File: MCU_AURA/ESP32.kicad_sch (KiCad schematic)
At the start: 15 parts, among them J2 TC2050-IDC-430, U200 ESP32-S3-WROOM-1, U201 USBLC6-2SC6

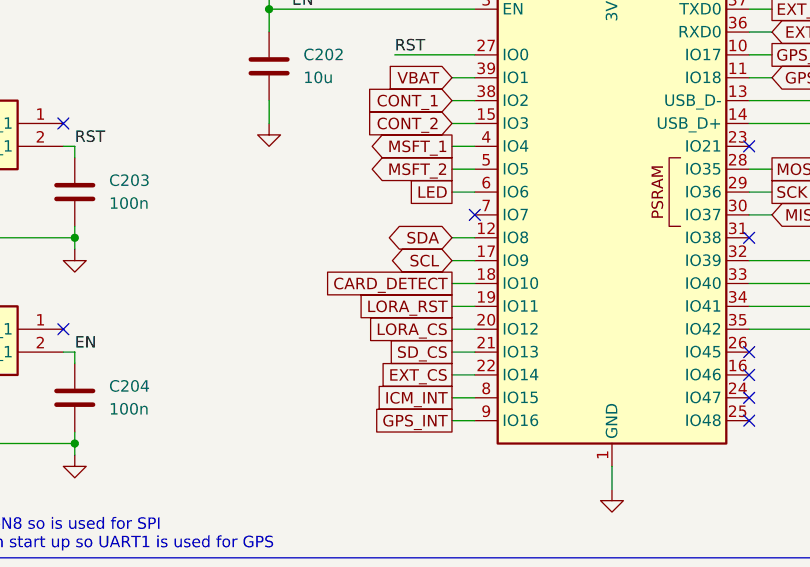
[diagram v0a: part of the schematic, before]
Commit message: Adding Connectors
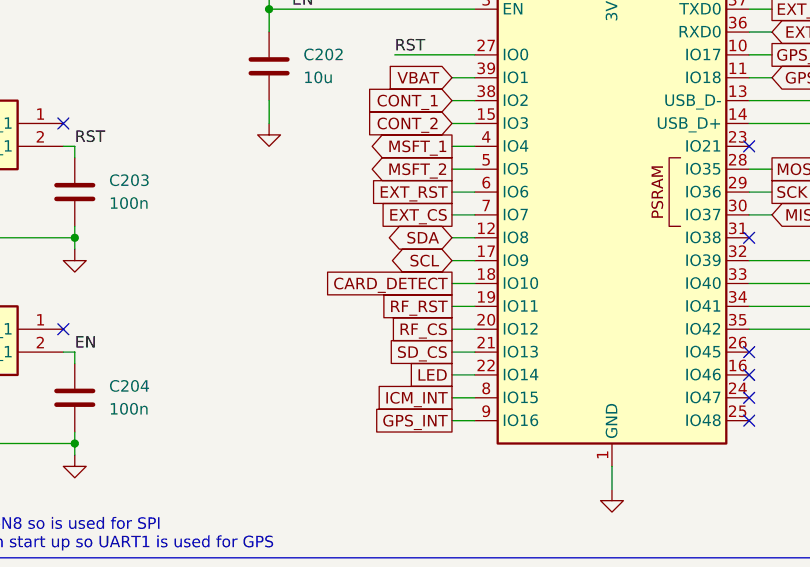
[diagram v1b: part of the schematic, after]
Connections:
- net EXT_CS: now also U200.7 (IO7); no longer U200.22 (IO14)
- net LED: now also U200.22 (IO14); no longer U200.6 (IO6)
- net LORA_CS renamed RF_CS
- net LORA_RST renamed RF_RST
- new net EXT_RST: U200.6 (IO6)
- no-connect marks 12 -> 11

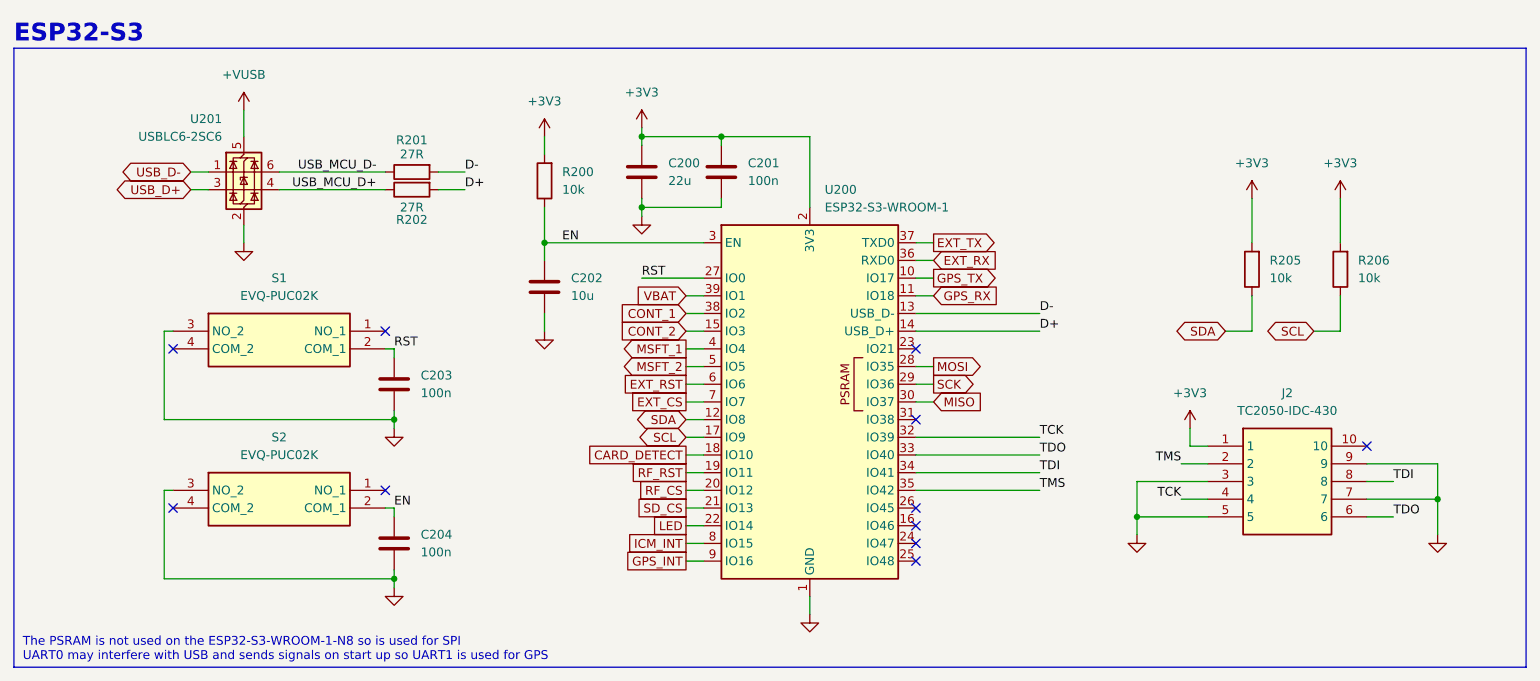
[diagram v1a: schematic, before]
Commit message: Initial Schematic Draft
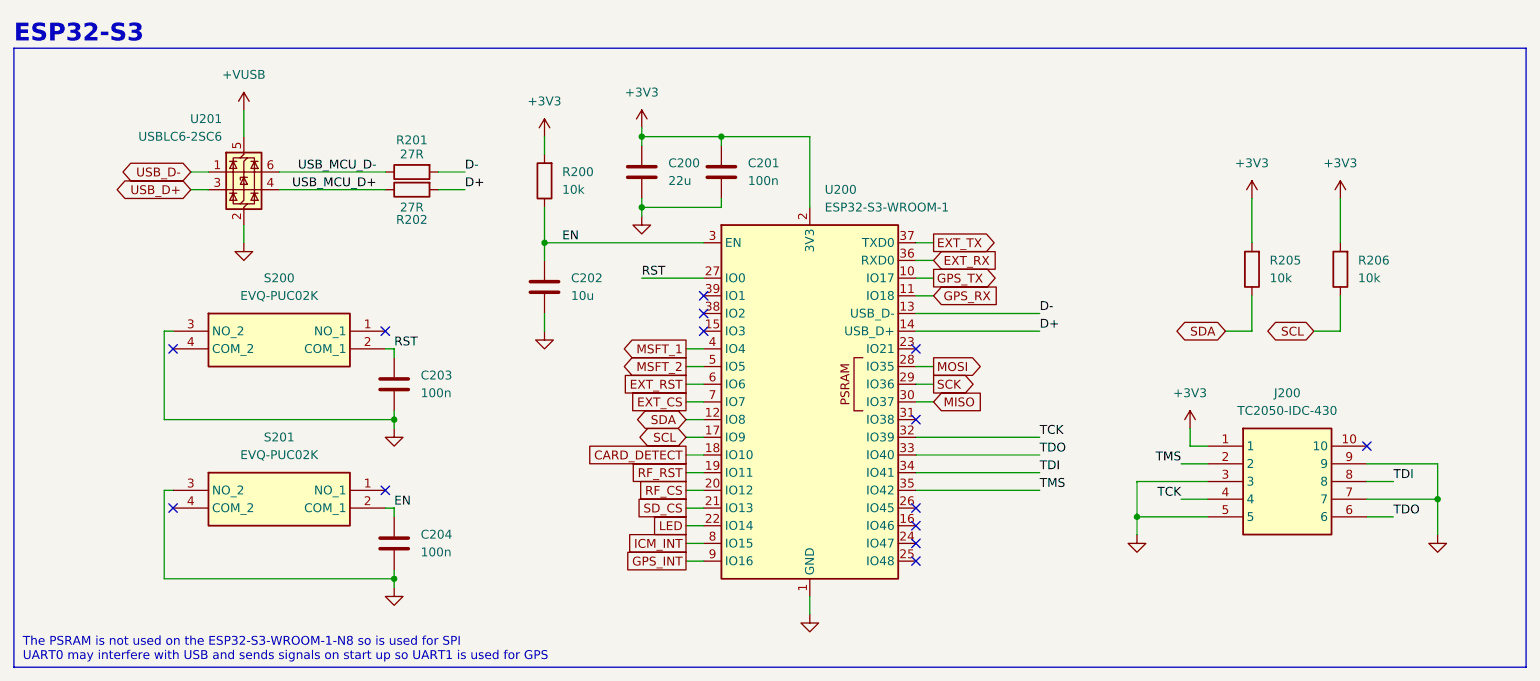
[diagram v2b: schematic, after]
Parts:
- renumbered J2 to J200, S1 to S200, S2 to S201
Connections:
- net CONT_1: no longer names the net of U200.38 (IO2)
- net CONT_2: no longer names the net of U200.15 (IO3)
- net VBAT: no longer names the net of U200.39 (IO1)
- no-connect marks 11 -> 14
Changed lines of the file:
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@@
 	)
 	(no_connect
+		(at 138.43 86.36)
+	)
+	(no_connect
+		(at 138.43 88.9)
+	)
+	(no_connect
 		(at 168.91 119.38)
 	)
@@
 	)
 	(no_connect
+		(at 138.43 91.44)
+	)
+	(no_connect
 		(at 168.91 104.14)
 	)
@@
 	(wire
 		(pts
-			(xy 135.89 91.44) (xy 138.43 91.44)
-		)
-		(stroke
-			(width 0)
-			(type default)
-		)
-	)
-	(wire
-		(pts
 			(xy 243.84 120.65) (xy 243.84 115.57)
 		)
@@
 	(wire
 		(pts
-			(xy 135.89 86.36) (xy 138.43 86.36)
-		)
-		(stroke
-			(width 0)
-			(type default)
-		)
-	)
-	(wire
-		(pts
-			(xy 135.89 88.9) (xy 138.43 88.9)
-		)
-		(stroke
-			(width 0)
-			(type default)
-		)
-	)
-	(wire
-		(pts
 			(xy 200.66 118.11) (xy 200.66 120.65)
 		)
@@
 		)
 	)
-	(global_label "CONT_1"
-		(shape input)
-		(at 135.89 88.9 180)
-		(fields_autoplaced yes)
-		(effects
-			(font
-				(size 1.27 1.27)
-			)
-			(justify right)
-		)
-		(property "Intersheetrefs" "${INTERSHEET_REFS}"
-			(at 125.8291 88.9 0)
-			(effects
-				(font
-					(size 1.27 1.27)
-				)
-				(justify right)
-				(hide yes)
-			)
-		)
-	)
 	(global_label "EXT_TX"
 		(shape output)
@@
 		)
 	)
-	(global_label "VBAT"
-		(shape input)
-		(at 135.89 86.36 180)
-		(fields_autoplaced yes)
-		(effects
-			(font
-				(size 1.27 1.27)
-			)
-			(justify right)
-		)
-		(property "Intersheetrefs" "${INTERSHEET_REFS}"
-			(at 128.49 86.36 0)
-			(effects
-				(font
-					(size 1.27 1.27)
-				)
-				(justify right)
-				(hide yes)
-			)
-		)
-	)
-	(global_label "CONT_2"
-		(shape input)
-		(at 135.89 91.44 180)
-		(fields_autoplaced yes)
-		(effects
-			(font
-				(size 1.27 1.27)
-			)
-			(justify right)
-		)
-		(property "Intersheetrefs" "${INTERSHEET_REFS}"
-			(at 125.8291 91.44 0)
-			(effects
-				(font
-					(size 1.27 1.27)
-				)
-				(justify right)
-				(hide yes)
-			)
-		)
-	)
 	(global_label "EXT_CS"
 		(shape passive)
@@
 		(dnp no)
 		(fields_autoplaced yes)
-		(property "Reference" "J2"
+		(property "Reference" "J200"
 			(at 222.25 100.33 0)
 			(effects
@@
 			(project ""
 				(path "/c0b09de1-c640-438f-9ef5-dda14a6aac71/b7286ff6-080d-4fe9-98ea-7dd25e1f4a61"
-					(reference "J2")
+					(reference "J200")
 					(unit 1)
 				)
@@
 		(dnp no)
 		(fields_autoplaced yes)
-		(property "Reference" "S1"
+		(property "Reference" "S200"
 			(at 77.47 83.82 0)
 			(effects
@@
 			(project ""
 				(path "/c0b09de1-c640-438f-9ef5-dda14a6aac71/b7286ff6-080d-4fe9-98ea-7dd25e1f4a61"
-					(reference "S1")
+					(reference "S200")
 					(unit 1)
 				)
@@
 		(dnp no)
 		(fields_autoplaced yes)
-		(property "Reference" "S2"
+		(property "Reference" "S201"
 			(at 77.47 106.68 0)
 			(effects
@@
 			(project "MCU_AURA"
 				(path "/c0b09de1-c640-438f-9ef5-dda14a6aac71/b7286ff6-080d-4fe9-98ea-7dd25e1f4a61"
-					(reference "S2")
+					(reference "S201")
 					(unit 1)
 				)

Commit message: Started Routing
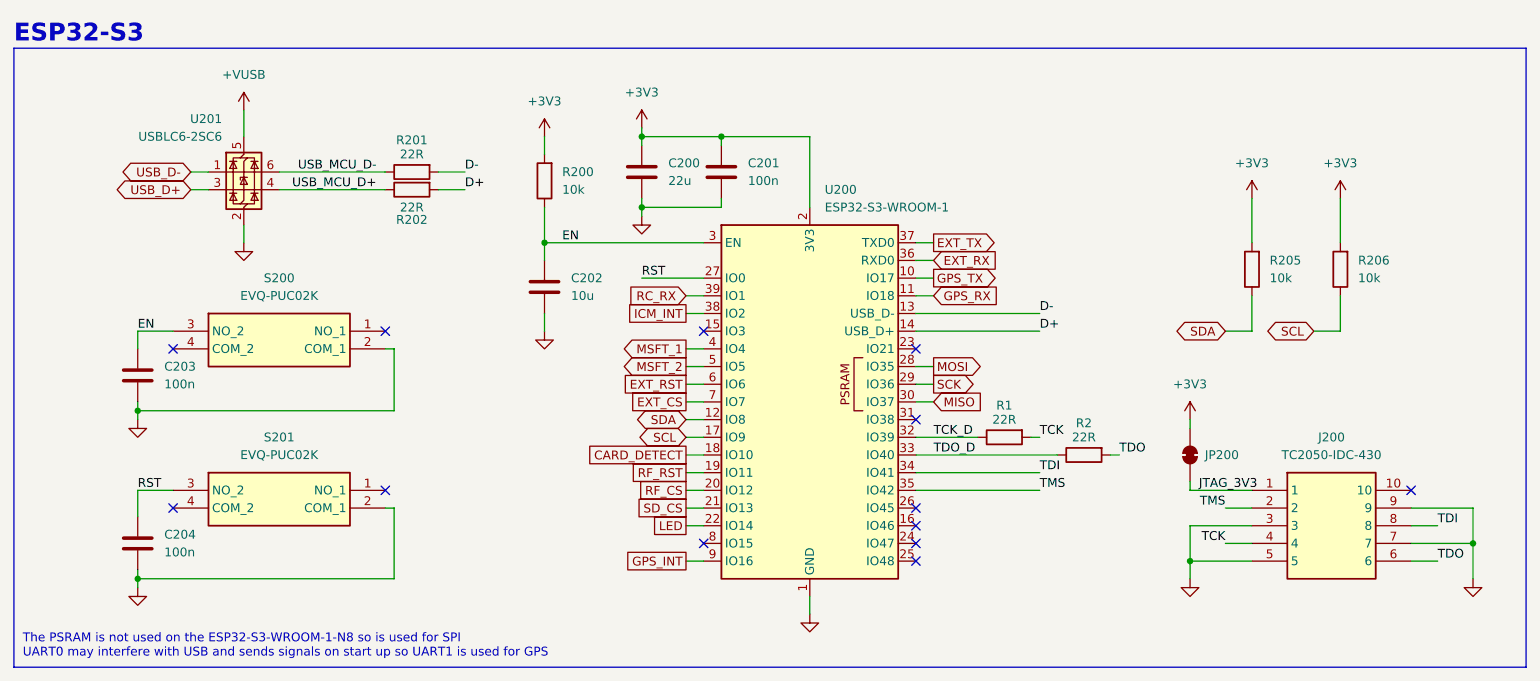
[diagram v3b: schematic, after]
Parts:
- added JP200: SolderJumper_2_Bridged, Jumper:SolderJumper-2_P1.3mm_Open_RoundedPad1.0x1.5mm, symbol Jumper:SolderJumper_2_Bridged
- added R1, R2: 22R, Resistor_SMD:R_0402_1005Metric, symbol Device:R
- J200: now left out of the parts list
- R201, R202: value 27R -> 22R
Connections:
- net +3V3: now also JP200.1 (A); no longer J200.1
- net EN: now also C203.1, S200.3 (NO_2); no longer C204.1, S201.2 (COM_1)
- net GND: now also S200.2 (COM_1), S201.2 (COM_1); no longer S200.3 (NO_2), S201.3 (NO_2)
- net ICM_INT: now also U200.38 (IO2); no longer U200.8 (IO15)
- net RST: now also C204.1, S201.3 (NO_2); no longer C203.1, S200.2 (COM_1)
- net TCK: now also R1.2; no longer U200.32 (IO39)
- net TDO: now also R2.2; no longer U200.33 (IO40)
- net RC_RX: now reaches U200.39 (IO1)
- new net JTAG_3V3: J200.1, JP200.2 (B)
- new net TCK_D: R1.1, U200.32 (IO39)
- new net TDO_D: R2.1, U200.33 (IO40)
- no-connect marks 14 -> 13
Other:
- moved on the sheet: C203, C204, J200

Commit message: First fully routed version
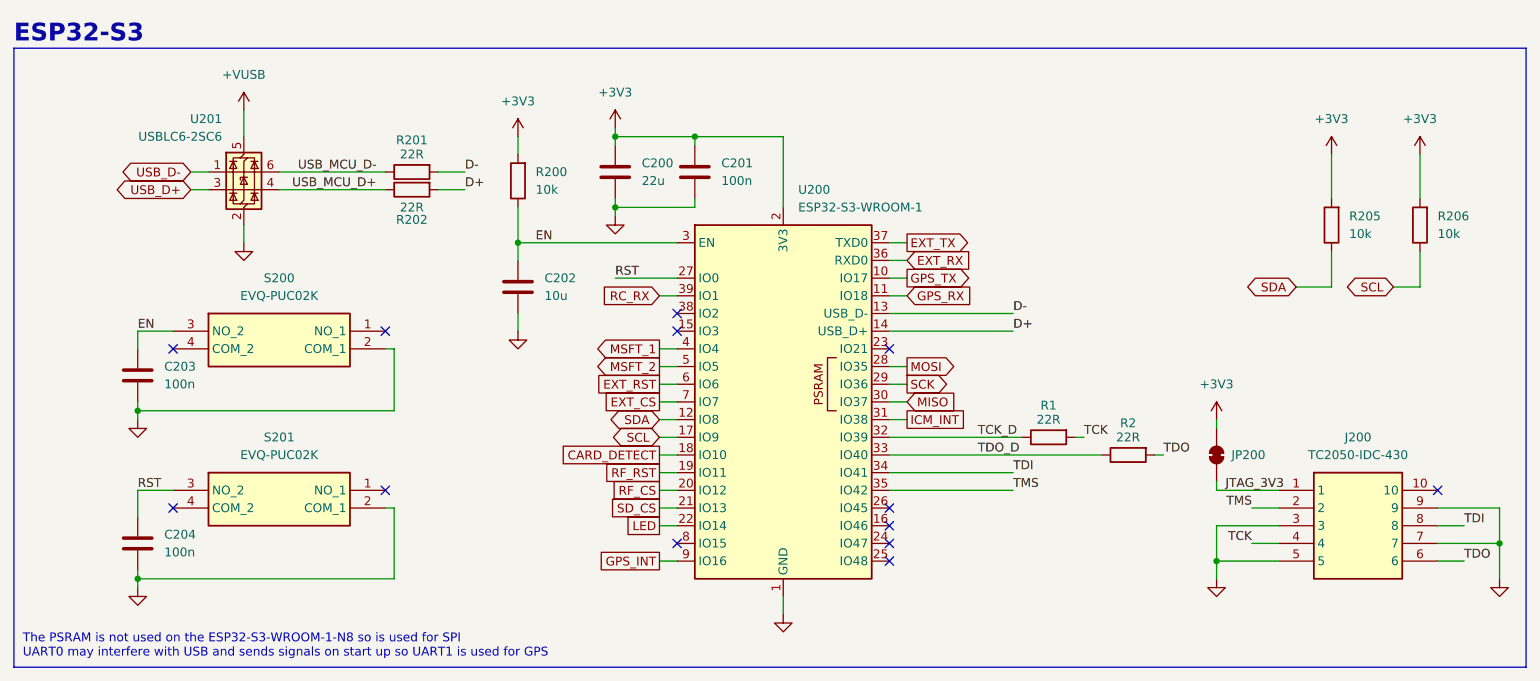
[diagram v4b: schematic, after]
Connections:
- net ICM_INT: now also U200.31 (IO38); no longer U200.38 (IO2)
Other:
- moved on the sheet: C200, C201, C202, J200, JP200, R1, R2, R200, R205, R206, U200
